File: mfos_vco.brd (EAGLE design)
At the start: 100 x 81.5 mm, 60 parts, among them IC1 TL072P, IC2 TL072P, IC3 TL072P, T1 2N3904, T2 2N3904, U1 POWER, U2 2N5457

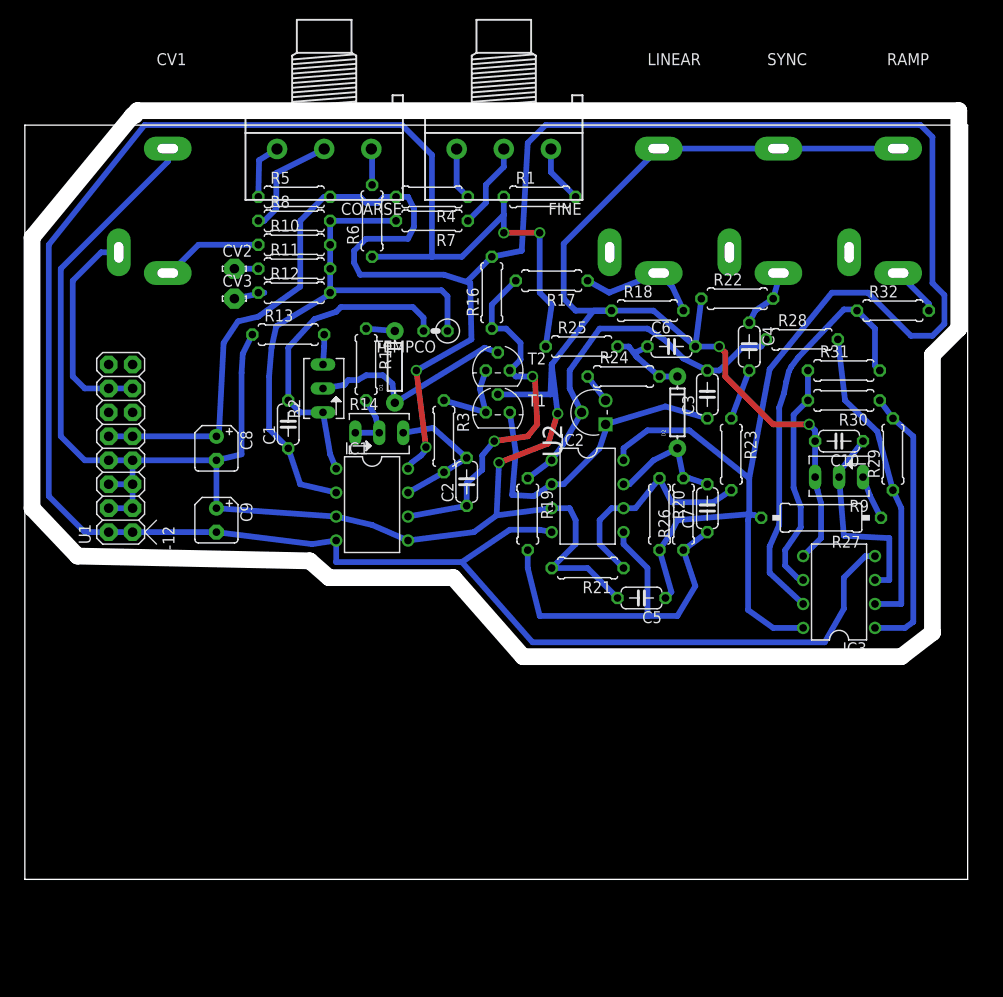
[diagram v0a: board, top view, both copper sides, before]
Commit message: same problem
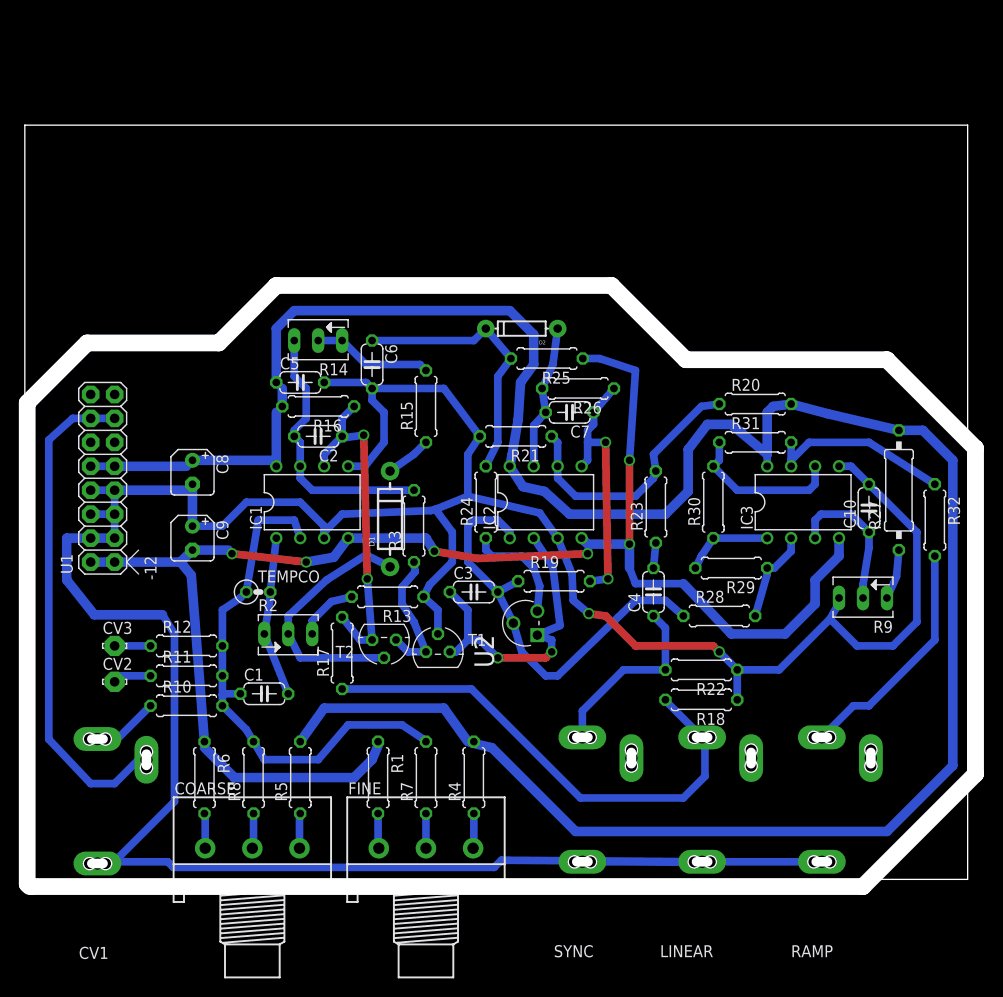
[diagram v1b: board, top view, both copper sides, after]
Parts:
- D1: device SparkFun-DiscreteSemi:DIODE-1N4148 -> SparkFun-DiscreteSemi:DIODE-1N4001
- R14: value 100k -> 20k
- moved LINEAR 82.0 mm to (76.8, -0.64), turned to 180 degrees
- moved SYNC 81.4 mm to (64.1, -0.64), turned to 180 degrees
- moved CV1 80.9 mm to (12.7, -0.81), turned to 180 degrees
- moved RAMP 80.7 mm to (89.5, -0.64), turned to 180 degrees
- moved FINE 74.6 mm to (42.5, 3.30), turned to 0 degrees
- moved COARSE 74.6 mm to (24.1, 3.30), turned to 0 degrees
- moved R1 63.9 mm to (37.5, 10.8), turned to 270 degrees
- moved R4 61.8 mm to (47.6, 10.8), turned to 90 degrees
- moved R6 61.7 mm to (19.1, 10.8), turned to 270 degrees
- moved R5 61.6 mm to (29.2, 10.8), turned to 90 degrees
- moved R8 59.2 mm to (24.3, 10.8), turned to 90 degrees
- moved R7 59.1 mm to (42.5, 10.8), turned to 90 degrees
- moved R10 50.2 mm to (17.1, 18.4)
- moved CV2 45.6 mm to (9.53, 21.0)
- moved R17 45.3 mm to (33.7, 24.0), turned to 90 degrees
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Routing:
- net -12V: track 233.9 -> 163.1 mm, vias 2 -> 6
- net GND: track 274.4 -> 341.2 mm, vias 4 -> 2
- net N$20: track 13.1 -> 54.1 mm
- net N$11: track 23.2 -> 53.0 mm
- net N$35: track 44.2 -> 20.5 mm
- net N$31: track 32.8 -> 9.93 mm
- net +12V: track 277.0 -> 256.3 mm, vias 2 -> 0
- net N$36: track 5.33 -> 25.2 mm
- net N$33: track 29.2 -> 9.42 mm
- net N$32: track 9.55 -> 28.9 mm
- net N$9: track 33.9 -> 17.1 mm
- net N$22: track 42.6 -> 27.9 mm, vias 0 -> 2
- net N$16: track 15.2 -> 28.5 mm
- net N$25: track 6.50 -> 19.7 mm
- net N$29: track 3.18 -> 11.8 mm
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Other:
- board size 100 x 81.5 mm -> 100.8 x 80.8 mm
